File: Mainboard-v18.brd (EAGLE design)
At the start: 50 x 50 mm, 37 parts, among them T1 2N3904, T2 2N3904

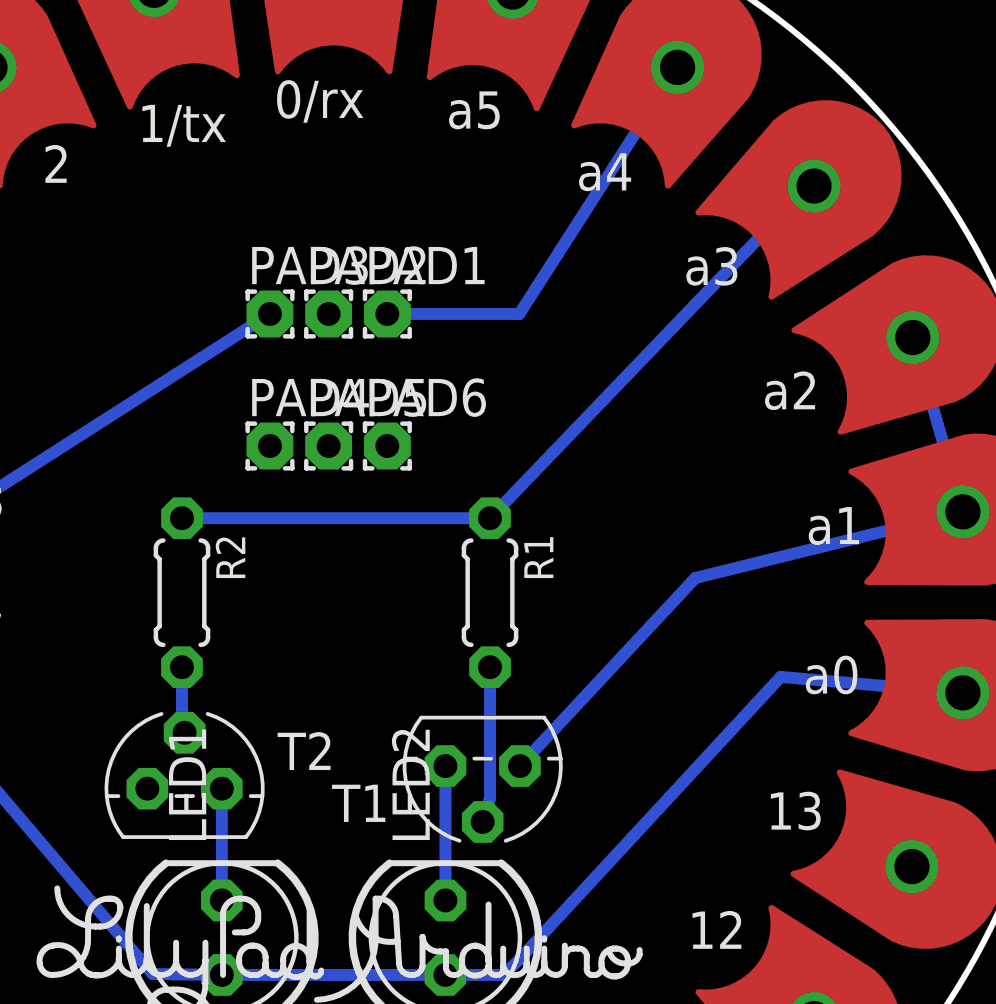
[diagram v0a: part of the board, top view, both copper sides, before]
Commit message: finish
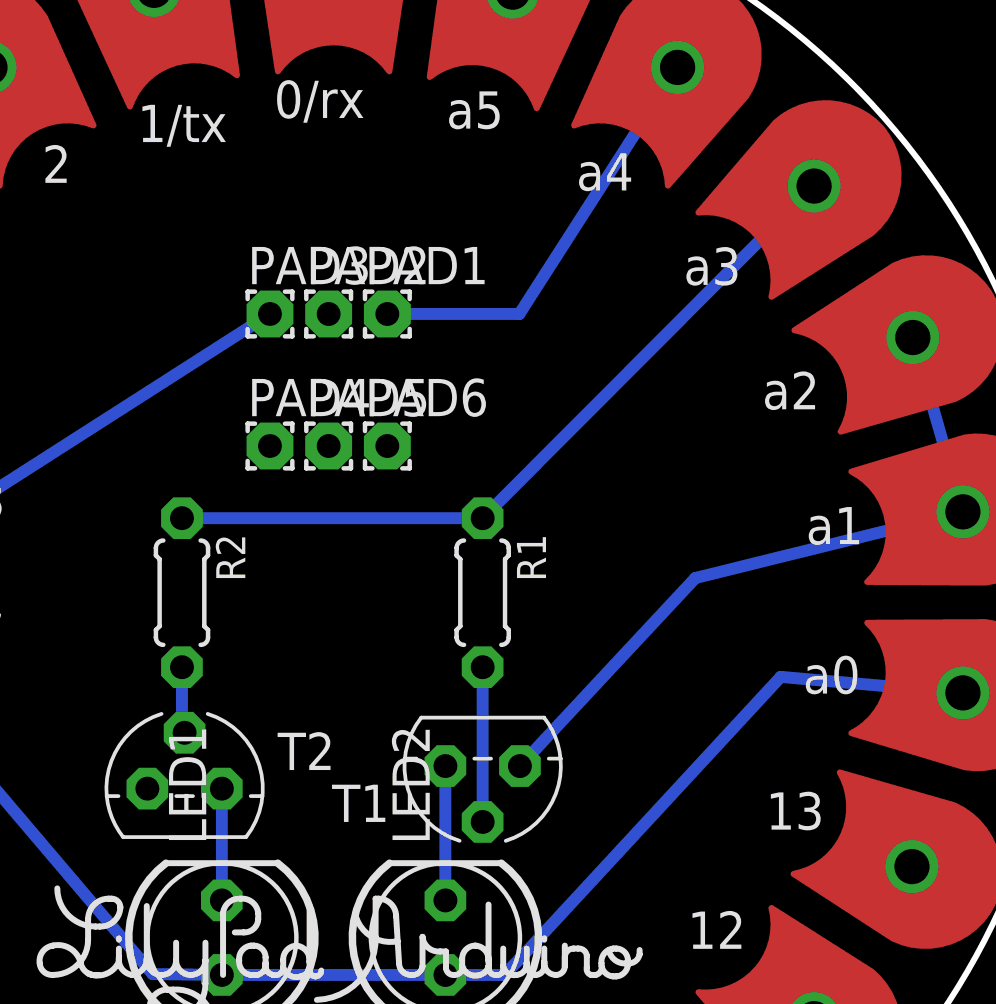
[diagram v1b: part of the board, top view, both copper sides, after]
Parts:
- moved R1 0.25 mm to (31.8, 27.0)
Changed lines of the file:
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@@
 <setting verticaltext="up"/>
 </settings>
-<grid distance="0.5" unitdist="mm" unit="mm" style="dots" multiple="1" display="yes" altdistance="0.1" altunitdist="mm" altunit="mm"/>
+<grid distance="0.25" unitdist="mm" unit="mm" style="dots" multiple="1" display="yes" altdistance="0.1" altunitdist="mm" altunit="mm"/>
 <layers>
 <layer number="1" name="Top" color="4" fill="1" visible="yes" active="yes"/>
@@
 <element name="PAD7" library="wirepad" package="1,6/0,8" value="" x="12" y="24"/>
 <element name="PAD8" library="wirepad" package="1,6/0,8" value="" x="12" y="28.5"/>
-<element name="R1" library="resistor" package="0204/5" value="" x="32" y="27" rot="R270"/>
+<element name="R1" library="resistor" package="0204/5" value="" x="31.75" y="27" rot="R270"/>
 <element name="R2" library="resistor" package="0204/5" value="" x="21.5" y="27" rot="R270"/>
 </elements>
@@
 <contactref element="R2" pad="1"/>
 <contactref element="R1" pad="1"/>
-<wire x1="43.047321875" y1="40.86035625" x2="43" y2="41" width="0.4064" layer="16"/>
-<wire x1="43" y1="41" x2="32" y2="29.54" width="0.4064" layer="16"/>
-<wire x1="32" y1="29.54" x2="21.5" y2="29.54" width="0.4064" layer="16"/>
+<wire x1="21.5" y1="29.54" x2="31.75" y2="29.54" width="0.4064" layer="16"/>
+<wire x1="43.047321875" y1="40.86035625" x2="31.75" y2="29.54" width="0.4064" layer="16"/>
 </signal>
 <signal name="A4">
@@
 <contactref element="T2" pad="2"/>
 <contactref element="R2" pad="2"/>
-<wire x1="21.5" y1="24.46" x2="21.5" y2="23" width="0.4064" layer="16"/>
-<wire x1="21.5" y1="23" x2="21.59" y2="22.225" width="0.4064" layer="16"/>
+<wire x1="21.5" y1="24.46" x2="21.5" y2="22.75" width="0.4064" layer="16"/>
+<wire x1="21.5" y1="22.75" x2="21.59" y2="22.225" width="0.4064" layer="16"/>
 </signal>
 <signal name="N$5">
 <contactref element="T1" pad="2"/>
 <contactref element="R1" pad="2"/>
-<wire x1="32" y1="24.46" x2="32" y2="20" width="0.4064" layer="16"/>
-<wire x1="32" y1="20" x2="31.75" y2="19.185" width="0.4064" layer="16"/>
+<wire x1="31.75" y1="24.46" x2="31.75" y2="19.185" width="0.4064" layer="16"/>
 </signal>
 </signals>
